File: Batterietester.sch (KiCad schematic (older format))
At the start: 16 parts, among them J1 CONN_01X02, J2 CONN_01X02, J3 CONN_01X02, J4 CONN_01X02, SW1 SW_Push, SW2 SW_Push, U1 LM3914

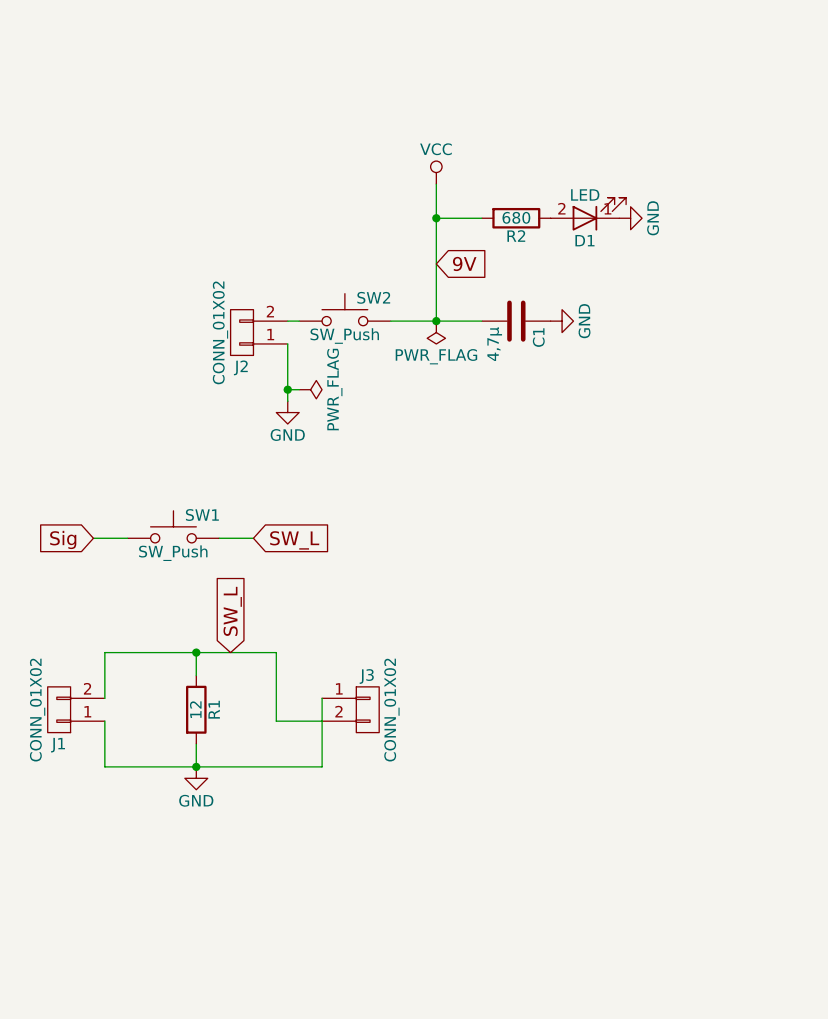
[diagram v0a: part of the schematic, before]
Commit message: cleaning
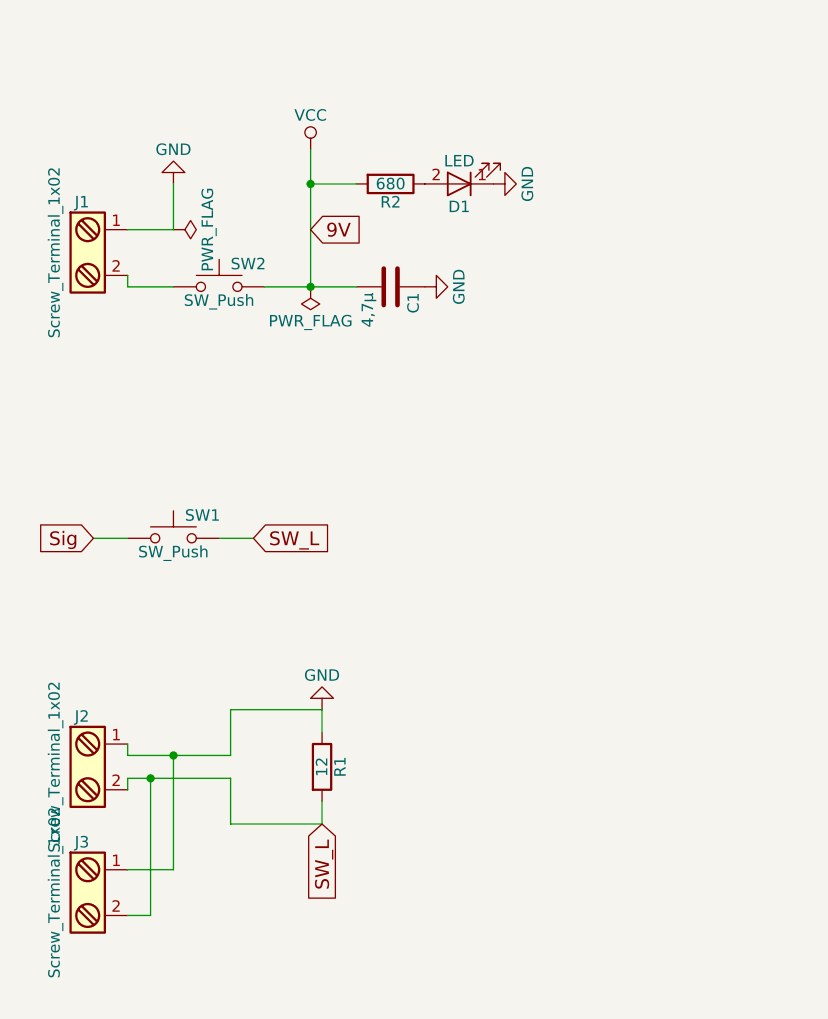
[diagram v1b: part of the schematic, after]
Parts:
- removed J1, J2, J3: CONN_01X02, Pin_Headers:Pin_Header_Angled_1x02_Pitch2.54mm, symbol CONN_01X02
- added J1, J2, J3: Screw_Terminal_1x02, TerminalBlock_Phoenix:TerminalBlock_Phoenix_MKDS1.5-2pol, symbol Screw_Terminal_1x02
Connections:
- net GND: now also R1.1, J1.1, J2.1, J3.1; no longer R1.2
- net SW_L: now also R1.2, J2.2, J3.2; no longer R1.1
- net at SW2.1: now also J1.2
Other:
- moved on the sheet: C1, D1, R1, R2, SW2
